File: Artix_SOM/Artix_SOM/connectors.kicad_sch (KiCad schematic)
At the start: 2 parts

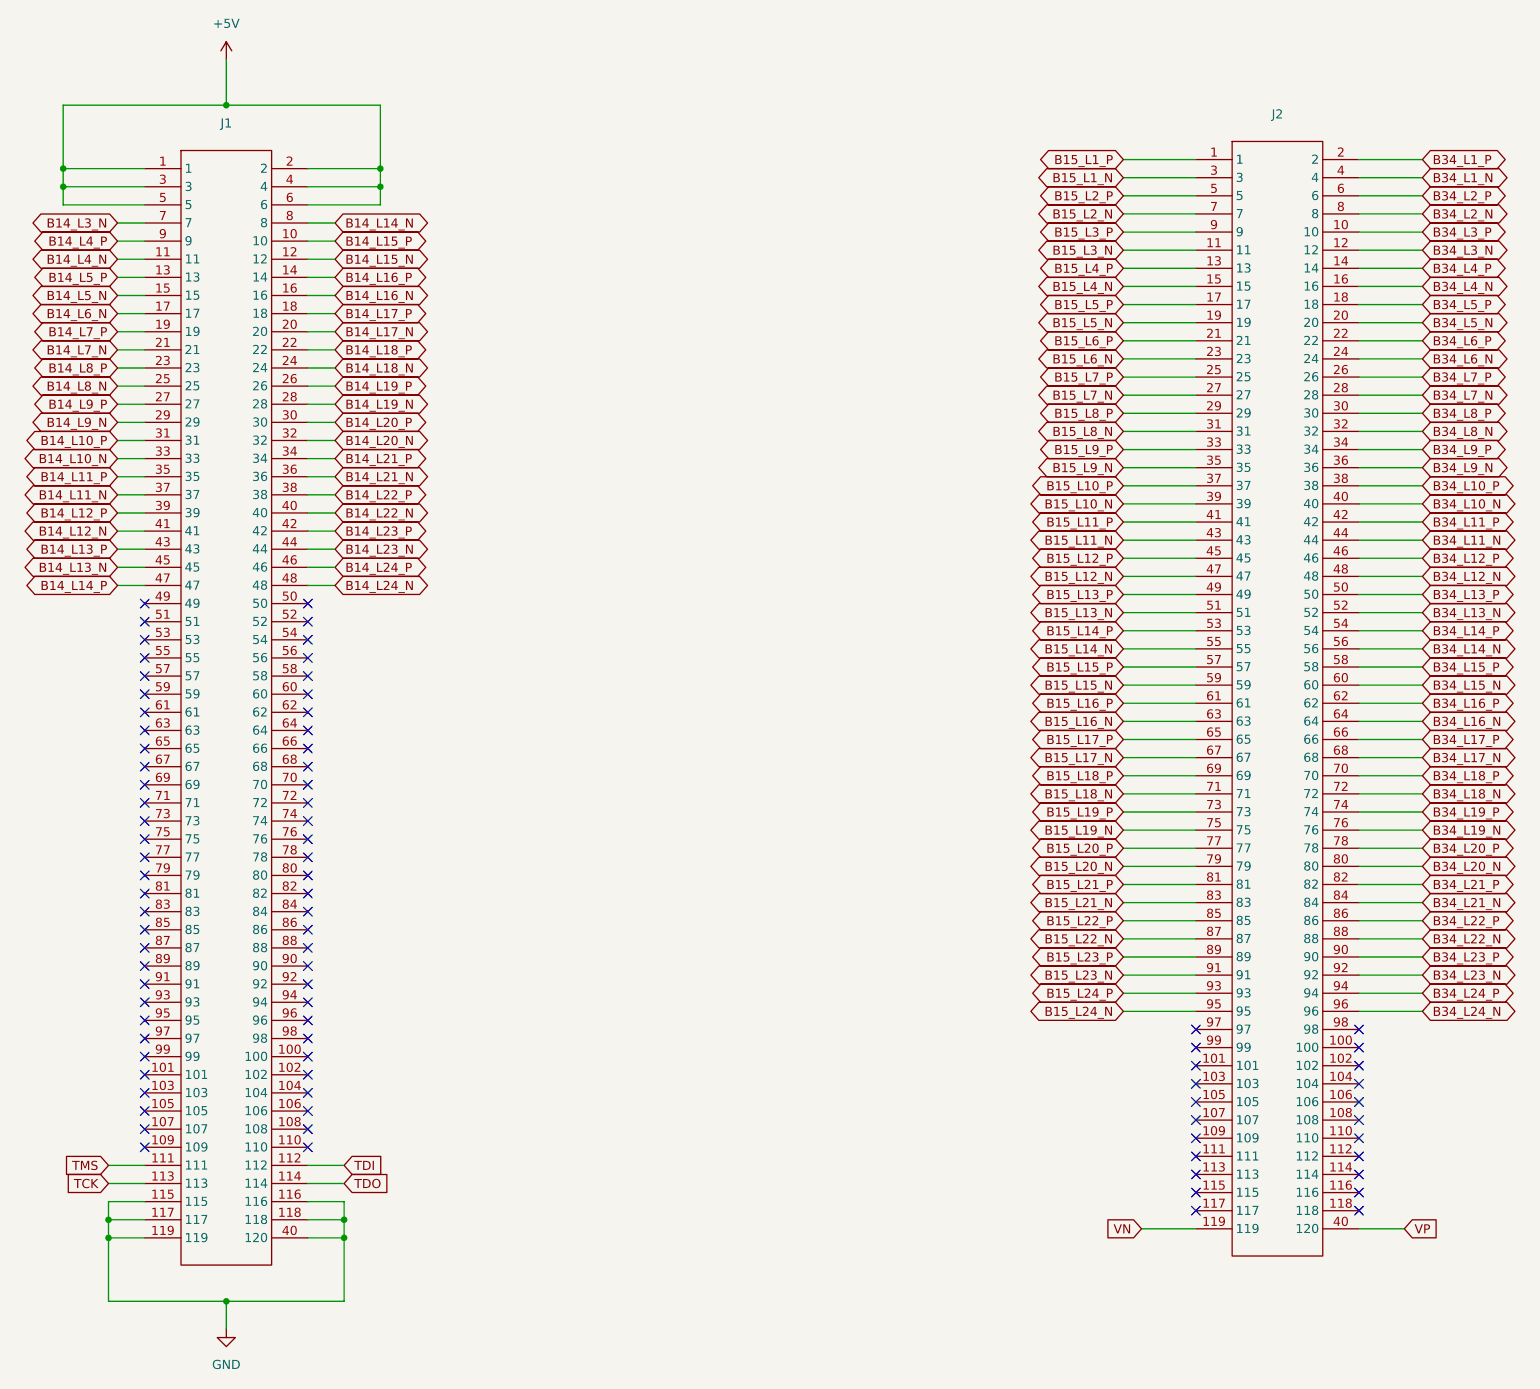
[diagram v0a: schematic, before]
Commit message: update
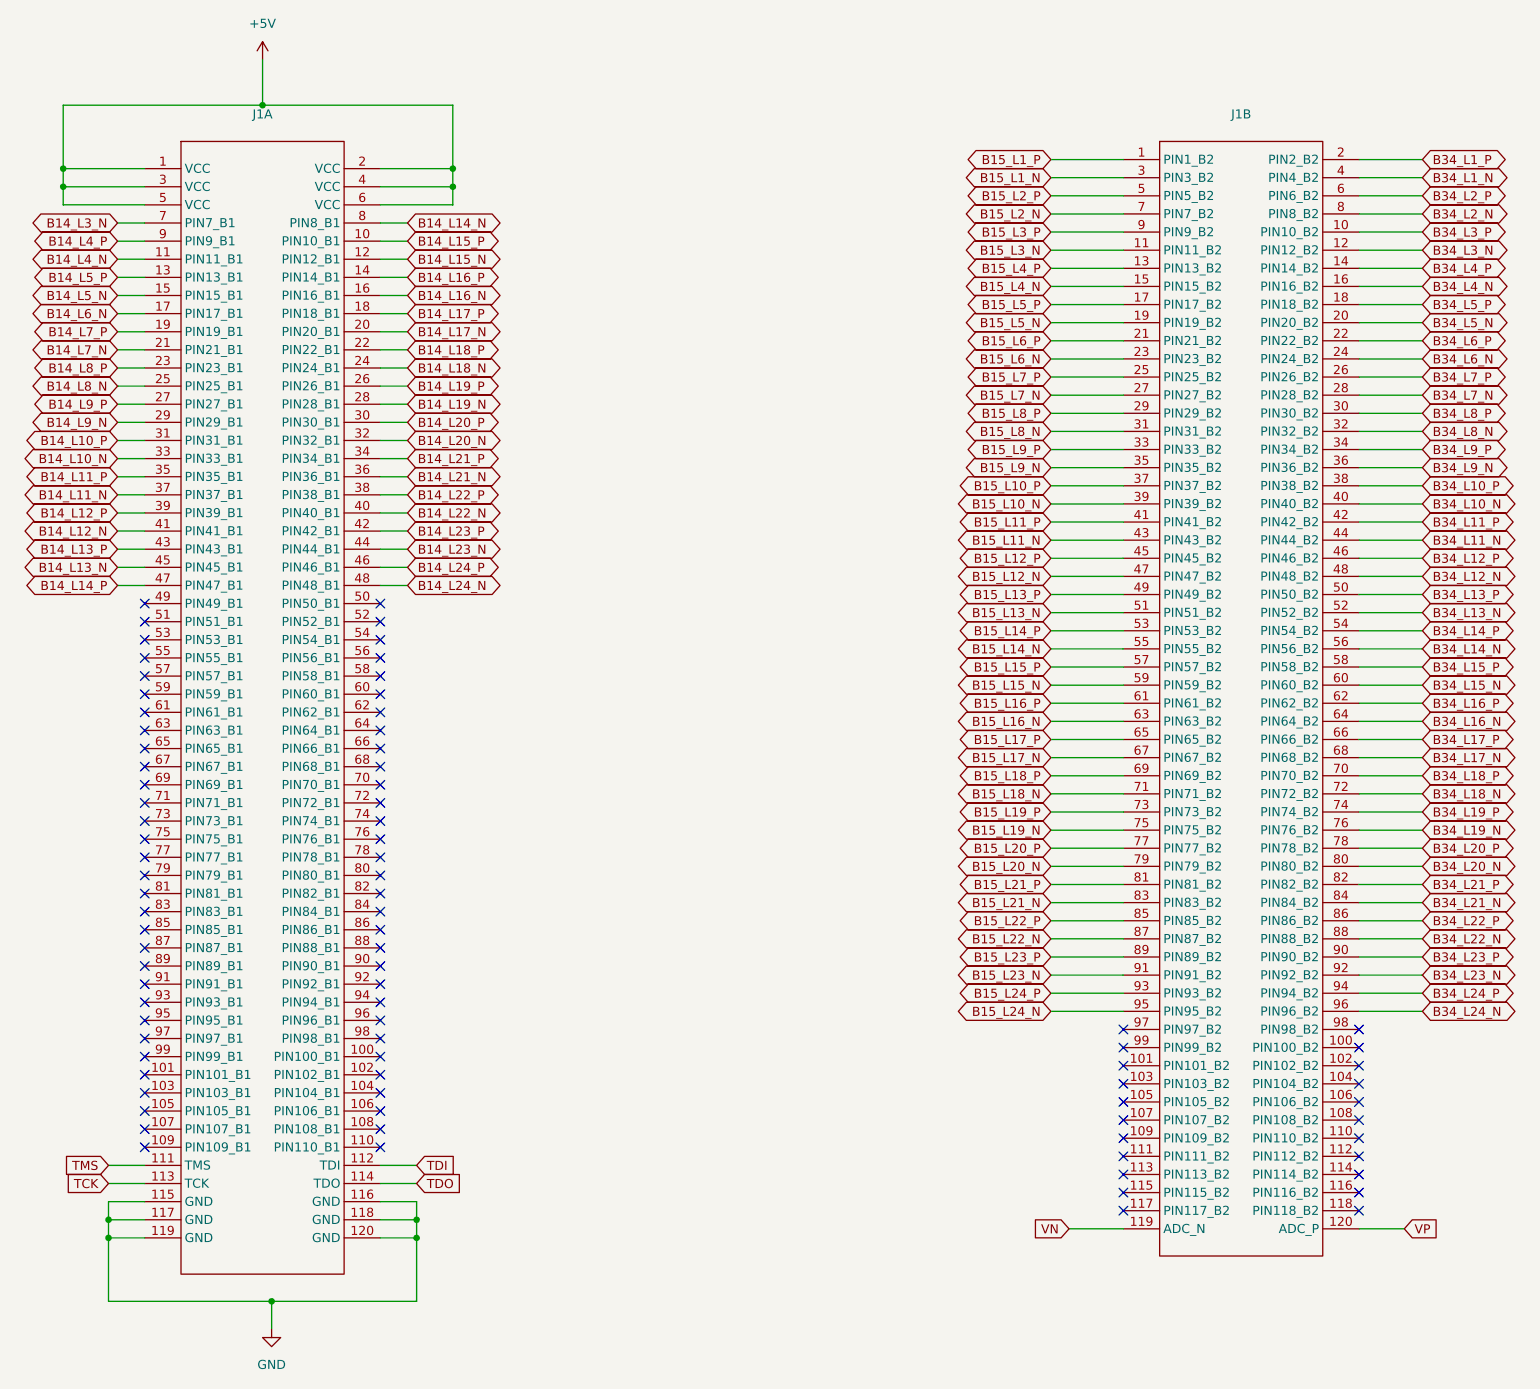
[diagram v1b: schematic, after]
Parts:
- removed J2: ~, symbol Panasonic_connector:AXK6A2337YG
- added unit 2 of J1
- J1: symbol Panasonic_connector:AXK6A2337YG -> SOM_library:SoM_male
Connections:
- net B15_L10_N: now also J1.39 (PIN39_B2)
- net B15_L10_P: now also J1.37 (PIN37_B2)
- net B15_L11_N: now also J1.43 (PIN43_B2)
- net B15_L11_P: now also J1.41 (PIN41_B2)
- net B15_L12_N: now also J1.47 (PIN47_B2)
- net B15_L12_P: now also J1.45 (PIN45_B2)
- net B15_L13_N: now also J1.51 (PIN51_B2)
- net B15_L13_P: now also J1.49 (PIN49_B2)
- net B15_L14_N: now also J1.55 (PIN55_B2)
- net B15_L14_P: now also J1.53 (PIN53_B2)
- net B15_L15_N: now also J1.59 (PIN59_B2)
- net B15_L15_P: now also J1.57 (PIN57_B2)
- net B15_L16_N: now also J1.63 (PIN63_B2)
- net B15_L16_P: now also J1.61 (PIN61_B2)
- net B15_L17_N: now also J1.67 (PIN67_B2)
- net B15_L17_P: now also J1.65 (PIN65_B2)
- net B15_L18_N: now also J1.71 (PIN71_B2)
- net B15_L18_P: now also J1.69 (PIN69_B2)
- net B15_L19_N: now also J1.75 (PIN75_B2)
- net B15_L19_P: now also J1.73 (PIN73_B2)
- net B15_L1_N: now also J1.3 (PIN3_B2)
- net B15_L1_P: now also J1.1 (PIN1_B2)
- net B15_L20_N: now also J1.79 (PIN79_B2)
- net B15_L20_P: now also J1.77 (PIN77_B2)
- net B15_L21_N: now also J1.83 (PIN83_B2)
- net B15_L21_P: now also J1.81 (PIN81_B2)
- net B15_L22_N: now also J1.87 (PIN87_B2)
- net B15_L22_P: now also J1.85 (PIN85_B2)
- net B15_L23_N: now also J1.91 (PIN91_B2)
- net B15_L23_P: now also J1.89 (PIN89_B2)
- net B15_L24_N: now also J1.95 (PIN95_B2)
- net B15_L24_P: now also J1.93 (PIN93_B2)
- net B15_L2_N: now also J1.7 (PIN7_B2)
- net B15_L2_P: now also J1.5 (PIN5_B2)
- net B15_L3_N: now also J1.11 (PIN11_B2)
- net B15_L3_P: now also J1.9 (PIN9_B2)
- net B15_L4_N: now also J1.15 (PIN15_B2)
- net B15_L4_P: now also J1.13 (PIN13_B2)
- net B15_L5_N: now also J1.19 (PIN19_B2)
- net B15_L5_P: now also J1.17 (PIN17_B2)
- net B15_L6_N: now also J1.23 (PIN23_B2)
- net B15_L6_P: now also J1.21 (PIN21_B2)
- net B15_L7_N: now also J1.27 (PIN27_B2)
- net B15_L7_P: now also J1.25 (PIN25_B2)
- net B15_L8_N: now also J1.31 (PIN31_B2)
- net B15_L8_P: now also J1.29 (PIN29_B2)
- net B15_L9_N: now also J1.35 (PIN35_B2)
- net B15_L9_P: now also J1.33 (PIN33_B2)
- net B34_L10_N: now also J1.40 (PIN40_B2)
- net B34_L10_P: now also J1.38 (PIN38_B2)
- net B34_L11_N: now also J1.44 (PIN44_B2)
- net B34_L11_P: now also J1.42 (PIN42_B2)
- net B34_L12_N: now also J1.48 (PIN48_B2)
- net B34_L12_P: now also J1.46 (PIN46_B2)
- net B34_L13_N: now also J1.52 (PIN52_B2)
- net B34_L13_P: now also J1.50 (PIN50_B2)
- net B34_L14_N: now also J1.56 (PIN56_B2)
- net B34_L14_P: now also J1.54 (PIN54_B2)
- net B34_L15_N: now also J1.60 (PIN60_B2)
- net B34_L15_P: now also J1.58 (PIN58_B2)
- net B34_L16_N: now also J1.64 (PIN64_B2)
- net B34_L16_P: now also J1.62 (PIN62_B2)
- net B34_L17_N: now also J1.68 (PIN68_B2)
- net B34_L17_P: now also J1.66 (PIN66_B2)
- net B34_L18_N: now also J1.72 (PIN72_B2)
- net B34_L18_P: now also J1.70 (PIN70_B2)
- net B34_L19_N: now also J1.76 (PIN76_B2)
- net B34_L19_P: now also J1.74 (PIN74_B2)
- net B34_L1_N: now also J1.4 (PIN4_B2)
- net B34_L1_P: now also J1.2 (PIN2_B2)
- net B34_L20_N: now also J1.80 (PIN80_B2)
- net B34_L20_P: now also J1.78 (PIN78_B2)
- net B34_L21_N: now also J1.84 (PIN84_B2)
- net B34_L21_P: now also J1.82 (PIN82_B2)
- net B34_L22_N: now also J1.88 (PIN88_B2)
- net B34_L22_P: now also J1.86 (PIN86_B2)
- net B34_L23_N: now also J1.92 (PIN92_B2)
- net B34_L23_P: now also J1.90 (PIN90_B2)
- net B34_L24_N: now also J1.96 (PIN96_B2)
- net B34_L24_P: now also J1.94 (PIN94_B2)
- net B34_L2_N: now also J1.8 (PIN8_B2)
- net B34_L2_P: now also J1.6 (PIN6_B2)
- net B34_L3_N: now also J1.12 (PIN12_B2)
- net B34_L3_P: now also J1.10 (PIN10_B2)
- net B34_L4_N: now also J1.16 (PIN16_B2)
- net B34_L4_P: now also J1.14 (PIN14_B2)
- net B34_L5_N: now also J1.20 (PIN20_B2)
- net B34_L5_P: now also J1.18 (PIN18_B2)
- net B34_L6_N: now also J1.24 (PIN24_B2)
- net B34_L6_P: now also J1.22 (PIN22_B2)
- net B34_L7_N: now also J1.28 (PIN28_B2)
- net B34_L7_P: now also J1.26 (PIN26_B2)
- net B34_L8_N: now also J1.32 (PIN32_B2)
- net B34_L8_P: now also J1.30 (PIN30_B2)
- net B34_L9_N: now also J1.36 (PIN36_B2)
- net B34_L9_P: now also J1.34 (PIN34_B2)
- net GND: now also J1.120 (GND); no longer J1.40
- net VN: now also J1.119 (ADC_N)
- net VP: now also J1.120 (ADC_P)
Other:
- moved on the sheet: J1A
